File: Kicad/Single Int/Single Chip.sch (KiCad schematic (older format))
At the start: 2 parts, among them J1 Raspberry_Pi_2_3, U1 8088_Min_Mode

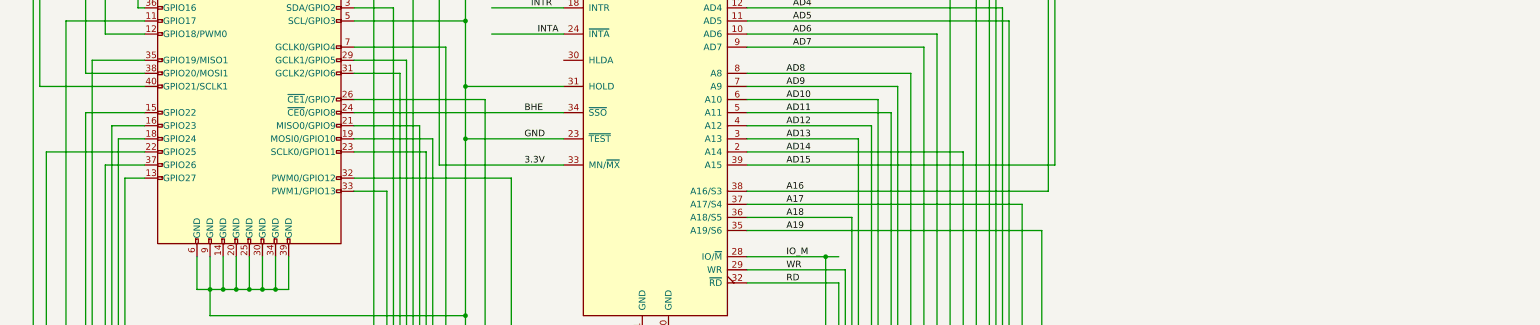
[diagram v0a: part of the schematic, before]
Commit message: Update PCB
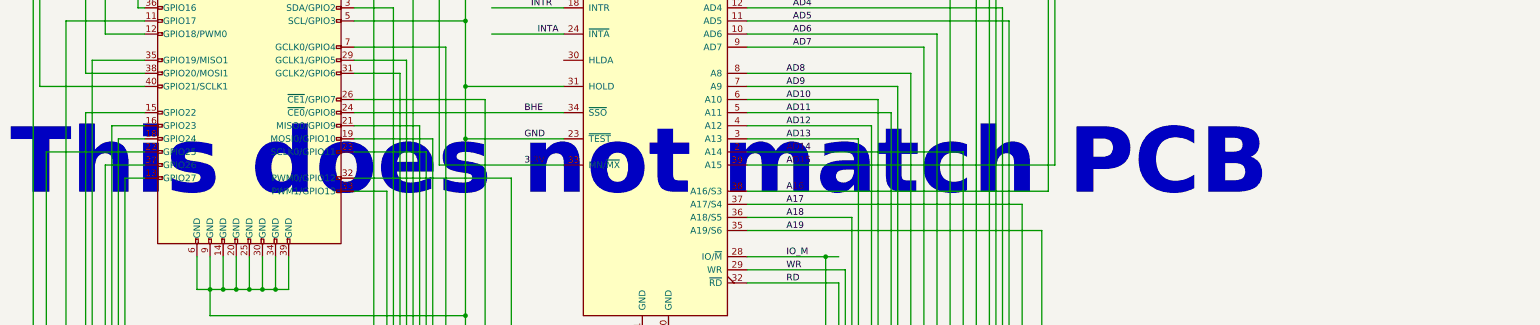
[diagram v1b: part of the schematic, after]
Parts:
- U1: footprint Package_DIP:DIP-40_W15.24mm -> Package_DIP:DIP-40_W15.24mm_LongPads
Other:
- note added: "This does not match PCB"
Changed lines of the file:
@@
 F 0 "U1" H 5550 5581 50  0000 C CNN
 F 1 "8088_Min_Mode" H 5550 5490 50  0000 C CNN
-F 2 "Package_DIP:DIP-40_W15.24mm" H 5600 3700 50  0001 C CIN
+F 2 "Package_DIP:DIP-40_W15.24mm_LongPads" H 5600 3700 50  0001 C CIN
 F 3 "http://datasheets.chipdb.org/Intel/x86/808x/datashts/8088/231456-006.pdf" H 5550 3650 50  0001 C CNN
 	1    5550 3600
@@
 Text Label 4650 3100 0    50   ~ 0
 INTA
+Text Notes 625  4375 0    500  ~ 100
+This does not match PCB
 $EndSCHEMATC

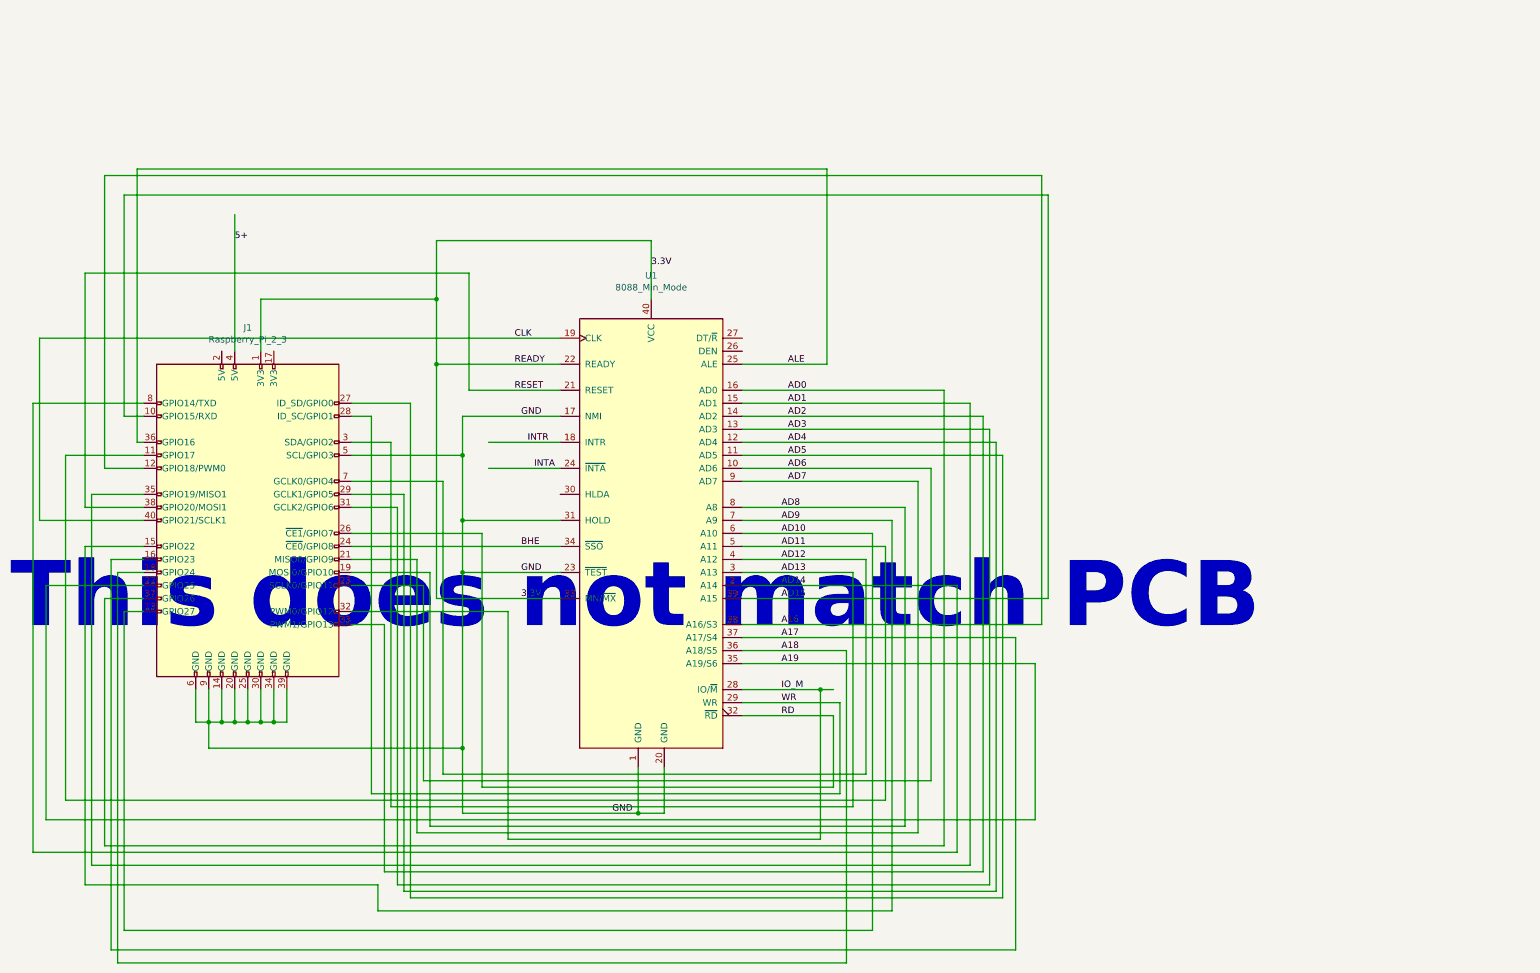
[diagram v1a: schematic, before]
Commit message: update
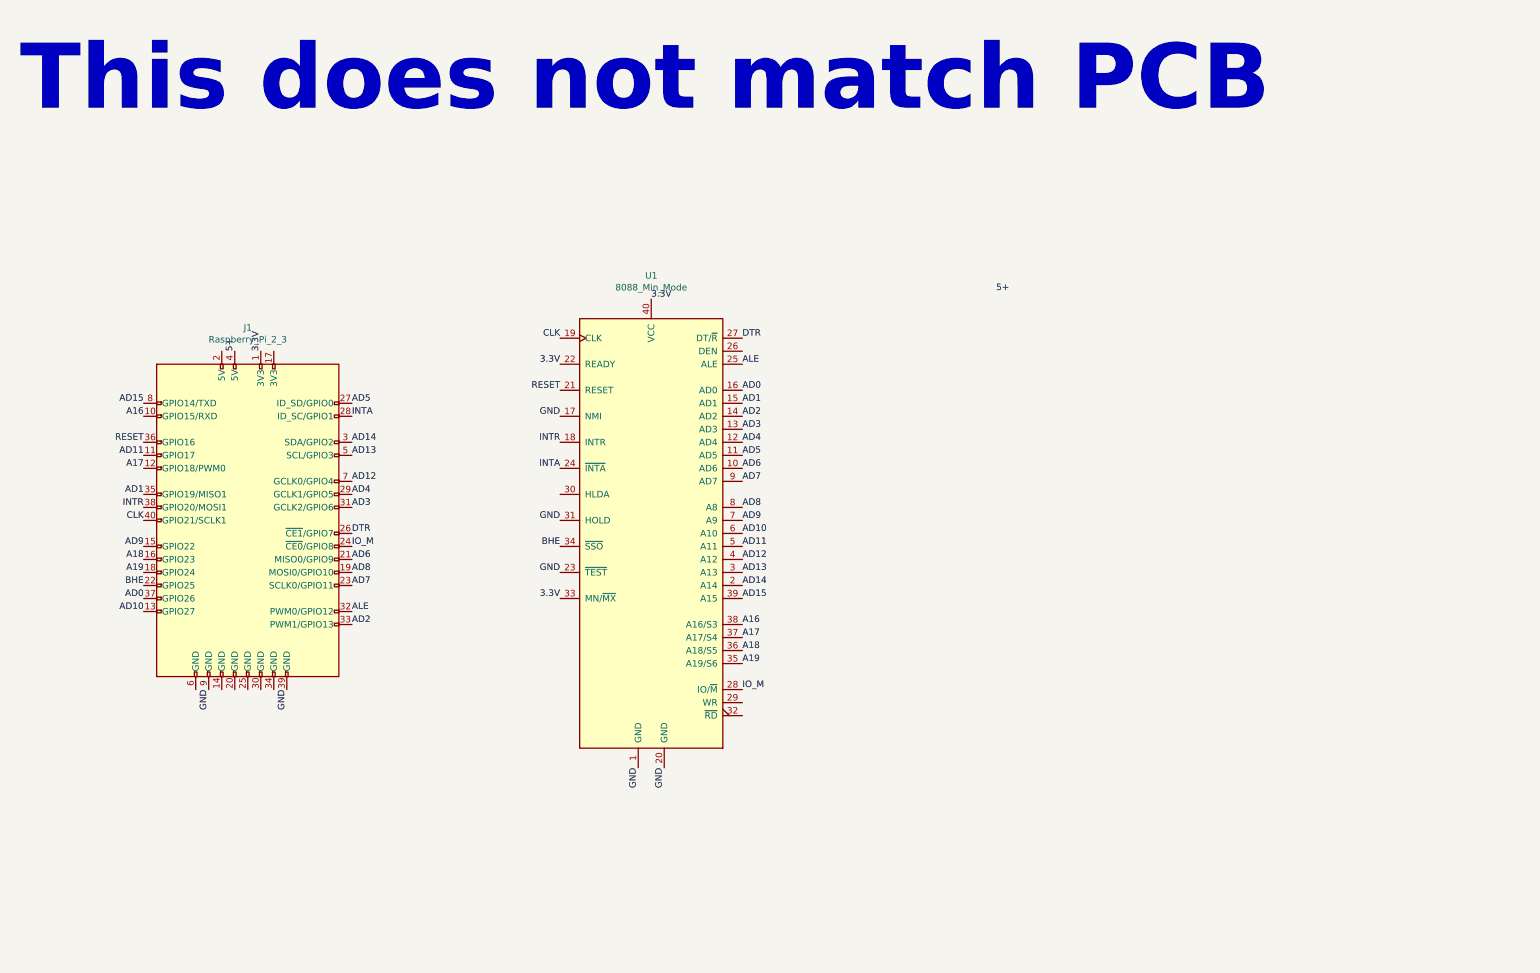
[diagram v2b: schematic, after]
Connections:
- net A16: now also J1.10 (GPIO15/RXD); no longer J1.12 (GPIO18/PWM0)
- net A17: now also J1.12 (GPIO18/PWM0); no longer J1.16 (GPIO23)
- net A18: now also J1.16 (GPIO23); no longer J1.18 (GPIO24)
- net A19: now also J1.18 (GPIO24); no longer J1.22 (GPIO25)
- net AD13: now also J1.5 (SCL/GPIO3); no longer J1.3 (SDA/GPIO2)
- net AD14: now also J1.3 (SDA/GPIO2); no longer J1.8 (GPIO14/TXD)
- net AD15: now also J1.8 (GPIO14/TXD); no longer J1.10 (GPIO15/RXD)
- net AD6: now also J1.21 (MISO0/GPIO9); no longer J1.23 (SCLK0/GPIO11)
- net AD7: now also J1.23 (SCLK0/GPIO11); no longer J1.21 (MISO0/GPIO9)
- net ALE: now also J1.32 (PWM0/GPIO12); no longer J1.36 (GPIO16)
- net BHE: now also J1.22 (GPIO25); no longer J1.24 (~CE0~/GPIO8)
- net GND: no longer J1.14 (GND), J1.20 (GND), J1.25 (GND), J1.30 (GND), J1.34 (GND), J1.5 (SCL/GPIO3), J1.6 (GND)
- net INTA: now also J1.28 (ID_SC/GPIO1)
- net INTR: now also J1.38 (GPIO20/MOSI1)
- net IO_M: now also J1.24 (~CE0~/GPIO8); no longer J1.32 (PWM0/GPIO12)
- net RESET: now also J1.36 (GPIO16); no longer J1.38 (GPIO20/MOSI1)
- net DTR: now reaches U1.27 (DT/~R~)
- net DTR: now also J1.26 (~CE1~/GPIO7)
- net RD: no longer names the net of U1.32 (~RD~)
- net RD: no longer J1.26 (~CE1~/GPIO7)
- net WR: no longer names the net of U1.29 (WR)
- net WR: no longer J1.28 (ID_SC/GPIO1)
